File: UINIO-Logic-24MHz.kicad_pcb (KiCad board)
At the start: 2 copper layers, 48.8 x 25.5 mm, 49 parts, among them J1 Conn_01x10_Pin, U1 AT24CS64-XHM, U2 74HC245C, U3 ME6211C33M5G-N, U4 CY7C68013A-56LTX, Y1 24MHz

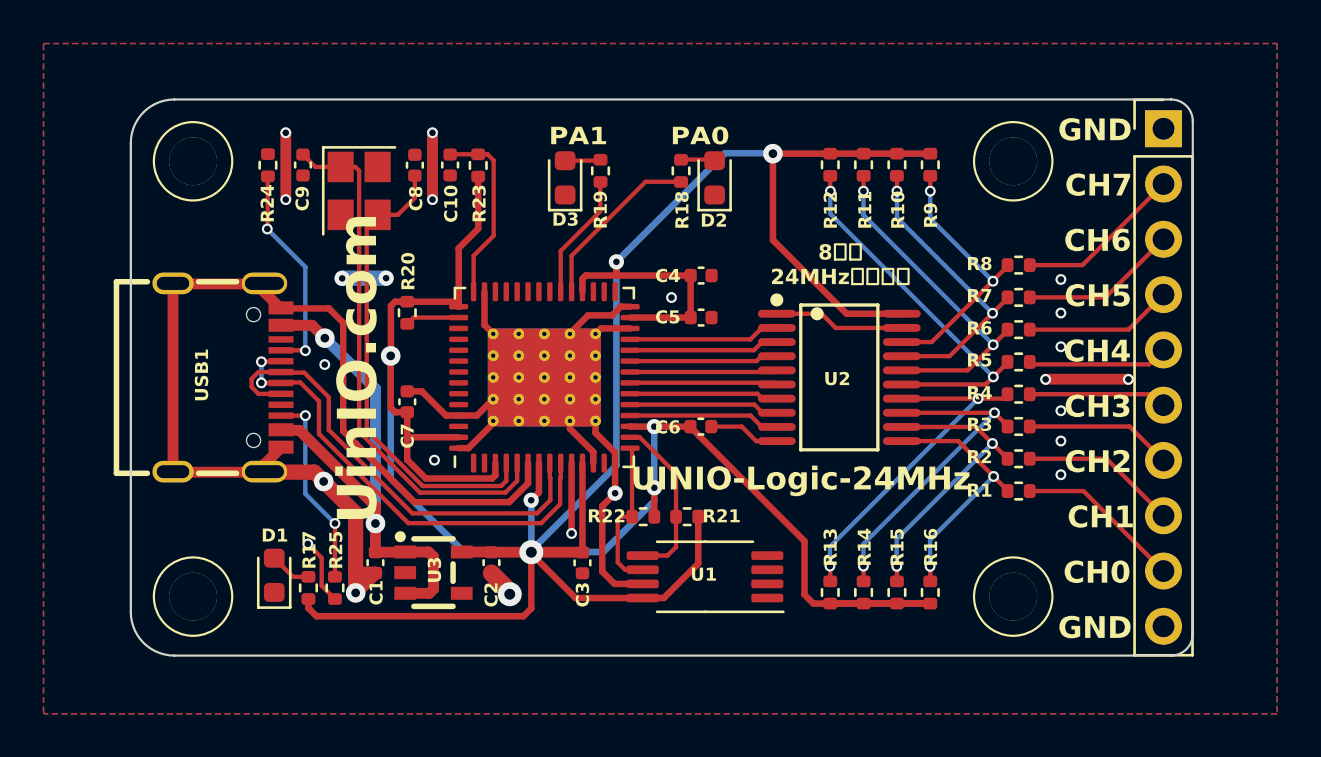
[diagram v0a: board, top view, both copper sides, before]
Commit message: Release UINIO-Logic-24MHz version 3.2.0.
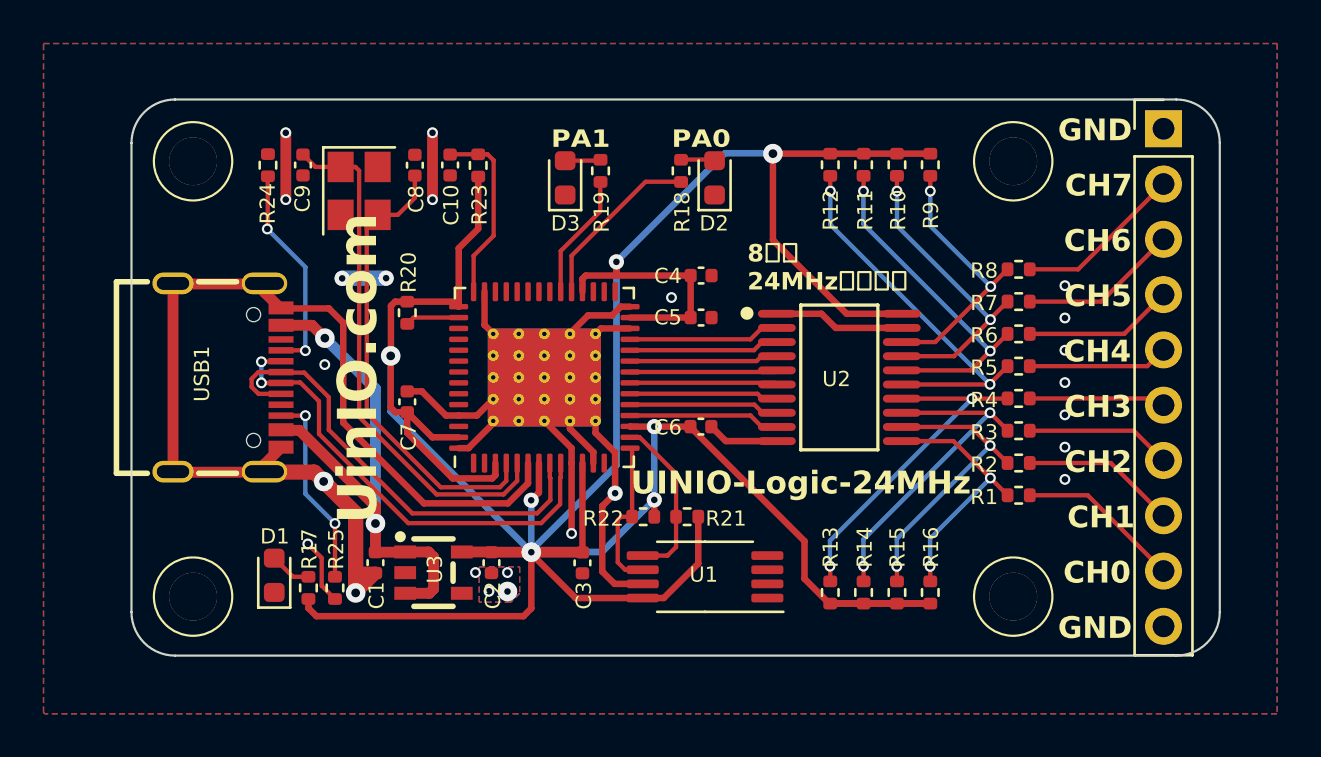
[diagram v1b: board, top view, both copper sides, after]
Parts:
- moved R3 0.19 mm to (167.4, 108.0)
- moved R4 0.19 mm to (167.4, 106.5)
- moved R6 0.19 mm to (167.4, 103.6)
- moved R7 0.19 mm to (167.4, 102.1)
- moved R1 0.19 mm to (167.4, 111.0)
- moved R2 0.19 mm to (167.4, 109.5)
- moved R5 0.19 mm to (167.4, 105.1)
- moved R8 0.19 mm to (167.4, 100.6)
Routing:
- net +3.3V: track 165.5 -> 162.4 mm
- net GND: track 104.8 -> 102.0 mm, vias 23 -> 24
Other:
- board size 48.8 x 25.5 mm -> 50 x 25.5 mm
- board text added: "Version 3.2.0"
- board text removed: "Version 3.1.1"
